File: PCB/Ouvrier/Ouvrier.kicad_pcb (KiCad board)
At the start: 2 copper layers, 8 parts, among them J1 Batterie, Q1 2N2222B, U1 XIAO-ESP32-S3-Plus-DIP, U2 BMP581, U3 UWB

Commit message: ouvrier
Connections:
- D1 pad 1: unconnected-(D1-K-Pad1) -> +3V3
- D1 pad 2: unconnected-(D1-A-Pad2) -> Net-(D1-A)
- J1 pad Bat+: unconnected-(J1-Pin_2-PadBat+) -> +3V3
- J1 pad Bat-: unconnected-(J1-Pin_1-PadBat-) -> GNDREF
- LS2 pad 1: unconnected-(LS2-+-Pad1) -> +3V3
- LS2 pad 2: unconnected-(LS2---Pad2) -> Net-(D1-A)
- Q1 pad 1: unconnected-(Q1-E-Pad1) -> GNDREF
- Q1 pad 2: unconnected-(Q1-B-Pad2) -> Net-(Q1-B)
- Q1 pad 3: unconnected-(Q1-C-Pad3) -> Net-(D1-A)
- R1 pad 1: unconnected-(R1-Pad1) -> Net-(U1-P0.28_A2_D2)
- R1 pad 2: unconnected-(R1-Pad2) -> Net-(Q1-B)
- U1 pad 3: unconnected-(U1-P0.28_A2_D2-Pad3) -> Net-(U1-P0.28_A2_D2)
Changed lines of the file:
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@@
 			(size 2.5 2.5)
 			(layers "F.Cu" "F.Mask" "F.Paste")
-			(net "unconnected-(LS2-+-Pad1)")
+			(net "+3V3")
 			(pinfunction "+_1")
 			(pintype "passive")
@@
 			(size 2.5 2.5)
 			(layers "F.Cu" "F.Mask" "F.Paste")
-			(net "unconnected-(LS2---Pad2)")
+			(net "Net-(D1-A)")
 			(pinfunction "-_2")
 			(pintype "passive")
@@
 			(remove_unused_layers no)
 			(roundrect_rratio 0.15)
-			(net "unconnected-(J1-Pin_2-PadBat+)")
+			(net "+3V3")
 			(pinfunction "Pin_2_Bat+")
 			(pintype "passive")
@@
 			(remove_unused_layers no)
 			(roundrect_rratio 0.15)
-			(net "unconnected-(J1-Pin_1-PadBat-)")
+			(net "GNDREF")
 			(pinfunction "Pin_1_Bat-")
 			(pintype "passive")
@@
 			(layers "F.Cu" "F.Mask")
 			(roundrect_rratio 0.1)
-			(net "unconnected-(U1-P0.28_A2_D2-Pad3)")
+			(net "Net-(U1-P0.28_A2_D2)")
 			(pinfunction "P0.28_A2_D2_3")
 			(pintype "passive")
@@
 			(layers "*.Cu" "*.Mask")
 			(remove_unused_layers no)
-			(net "unconnected-(U1-P0.28_A2_D2-Pad3)")
+			(net "Net-(U1-P0.28_A2_D2)")
 			(pinfunction "P0.28_A2_D2_3")
 			(pintype "passive")
@@
 			(remove_unused_layers no)
 			(roundrect_rratio 0.15625)
-			(net "unconnected-(D1-K-Pad1)")
+			(net "+3V3")
 			(pinfunction "K_1")
 			(pintype "passive")
@@
 			(layers "*.Cu" "*.Mask")
 			(remove_unused_layers no)
-			(net "unconnected-(D1-A-Pad2)")
+			(net "Net-(D1-A)")
 			(pinfunction "A_2")
 			(pintype "passive")
@@
 			(layers "*.Cu" "*.Mask")
 			(remove_unused_layers no)
-			(net "unconnected-(Q1-E-Pad1)")
+			(net "GNDREF")
 			(pinfunction "E_1")
 			(pintype "passive")
@@
 			(layers "*.Cu" "*.Mask")
 			(remove_unused_layers no)
-			(net "unconnected-(Q1-B-Pad2)")
+			(net "Net-(Q1-B)")
 			(pinfunction "B_2")
 			(pintype "passive")
@@
 			(layers "*.Cu" "*.Mask")
 			(remove_unused_layers no)
-			(net "unconnected-(Q1-C-Pad3)")
+			(net "Net-(D1-A)")
 			(pinfunction "C_3")
 			(pintype "passive")
@@
 			(layers "*.Cu" "*.Mask")
 			(remove_unused_layers no)
-			(net "unconnected-(R1-Pad1)")
+			(net "Net-(U1-P0.28_A2_D2)")
 			(pintype "passive")
 		)
@@
 			(layers "*.Cu" "*.Mask")
 			(remove_unused_layers no)
-			(net "unconnected-(R1-Pad2)")
-			(pintype "passive")
-		)
+			(net "Net-(Q1-B)")
+			(pintype "passive")
+		)

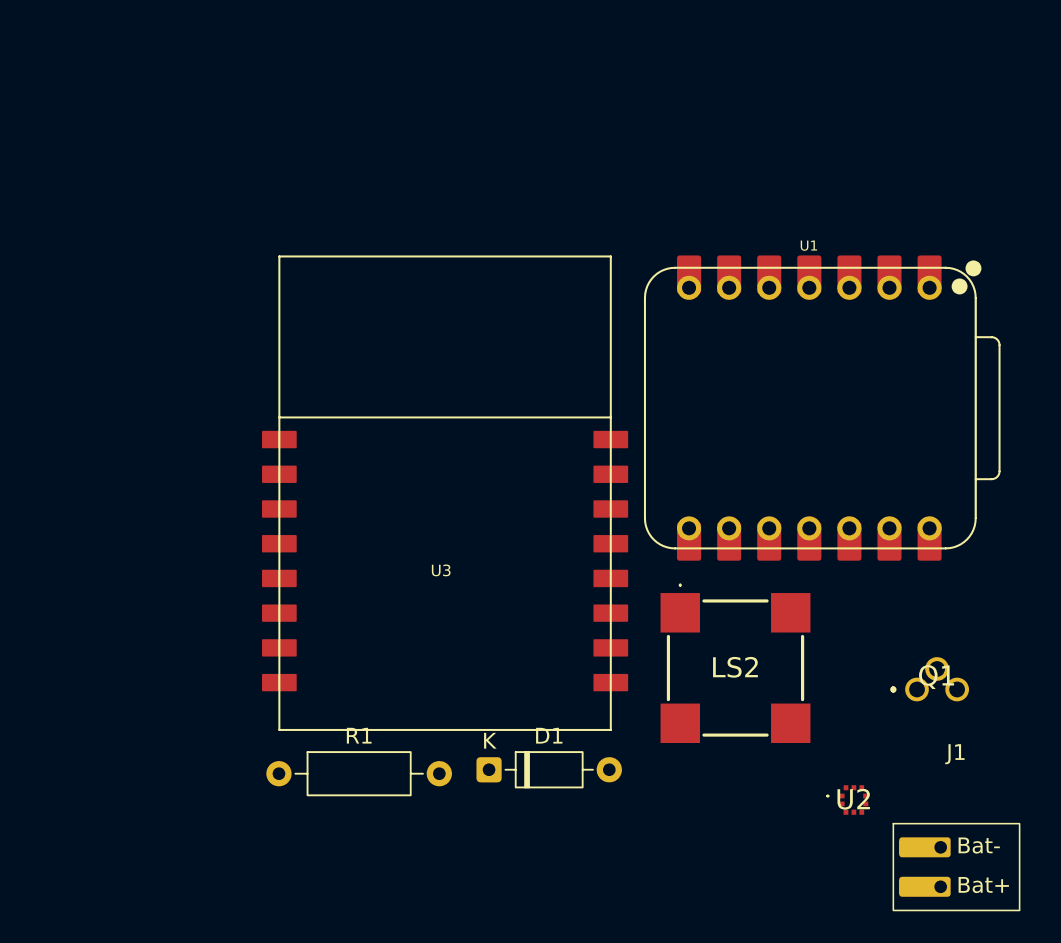
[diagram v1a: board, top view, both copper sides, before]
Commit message: Ouvrier_v2
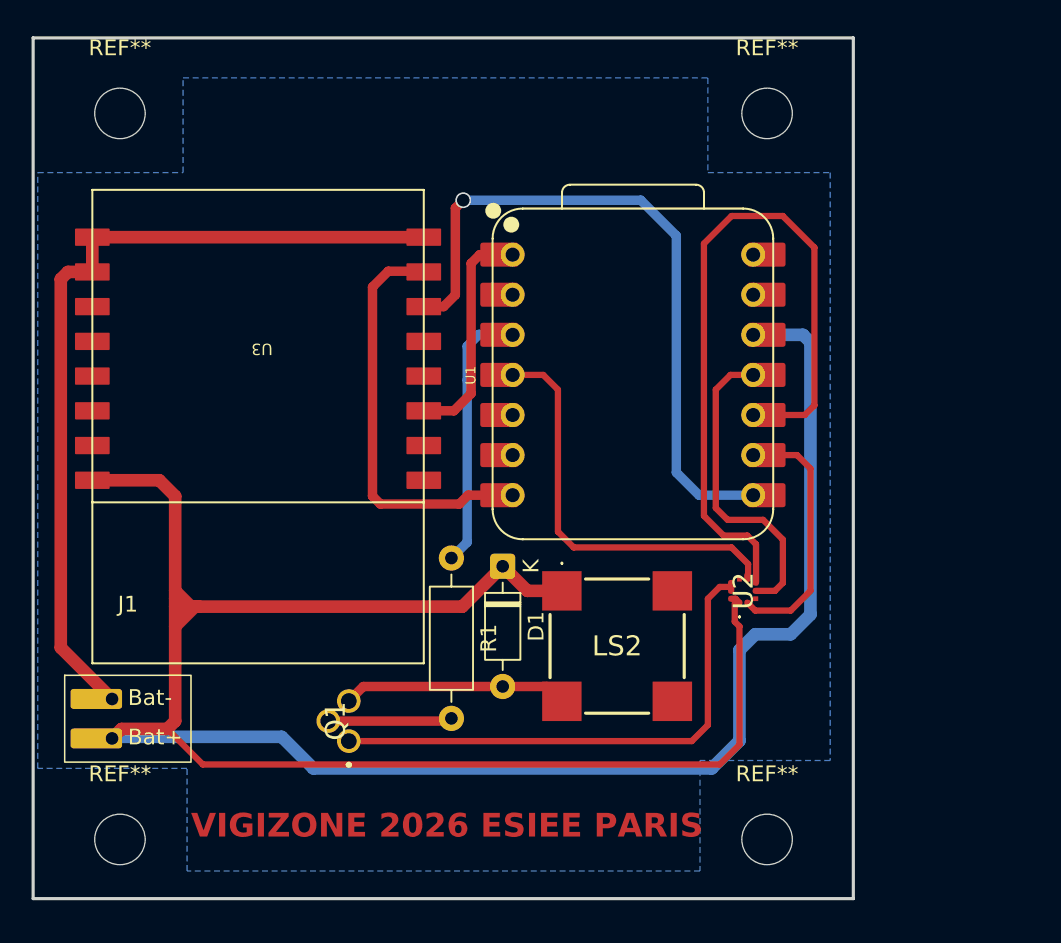
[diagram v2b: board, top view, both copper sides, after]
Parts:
- added REF**: MountingHole_3.2mm_M3, MountingHole:MountingHole_3.2mm_M3, F.Cu at (99.0, 106.0)
- added REF**: MountingHole_3.2mm_M3, MountingHole:MountingHole_3.2mm_M3, F.Cu at (140.0, 60.0)
- added REF**: MountingHole_3.2mm_M3, MountingHole:MountingHole_3.2mm_M3, F.Cu at (99.0, 60.0)
- added REF**: MountingHole_3.2mm_M3, MountingHole:MountingHole_3.2mm_M3, F.Cu at (140.0, 106.0)
- moved J1 53.3 mm to (99.5, 91.6)
- moved Q1 36.1 mm to (113.5, 99.8), turned to 90 degrees
- moved U3 35.4 mm to (118.2, 64.8), turned to 180 degrees
- moved R1 17.5 mm to (120.0, 88.2), turned to -90 degrees
- moved U2 15.0 mm to (138.5, 90.2), turned to 90 degrees
- moved D1 12.9 mm to (123.2, 88.7), turned to -90 degrees
- moved U1 11.4 mm to (131.5, 76.6), turned to 90 degrees
- moved LS2 7.63 mm to (130.5, 93.8)
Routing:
- net +3V3: track 0.00 -> 176.0 mm
- net GNDREF: track 0.00 -> 86.8 mm
- net Net-(U1-P1.14_D9_MISO): track 0.00 -> 45.6 mm
- net Net-(U1-P1.12_D7_RX): track 0.00 -> 43.4 mm, vias 0 -> 1
- net Net-(U1-P0.29_A3_D3): track 0.00 -> 26.9 mm
- net Net-(U1-P1.11_D6_TX): track 0.00 -> 26.3 mm
- net Net-(U1-P1.15_D10_MOSI): track 0.00 -> 20.0 mm
- net Net-(U1-P0.28_A2_D2): track 0.00 -> 17.0 mm
- net Net-(U1-P1.13_D8_SCK): track 0.00 -> 16.5 mm
- net Net-(D1-A): track 0.00 -> 14.3 mm
- net Net-(U1-P0.02_A0_D0): track 0.00 -> 13.7 mm
- net Net-(Q1-B): track 0.00 -> 7.87 mm
- added copper zone on B.Cu, net GNDREF
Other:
- board outline added: 52 x 54.5 mm
- board text added: "VIGIZONE 2026 ESIEE PARIS"
